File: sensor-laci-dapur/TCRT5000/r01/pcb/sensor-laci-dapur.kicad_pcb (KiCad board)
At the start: 2 copper layers, 66 x 14 mm, 8 parts

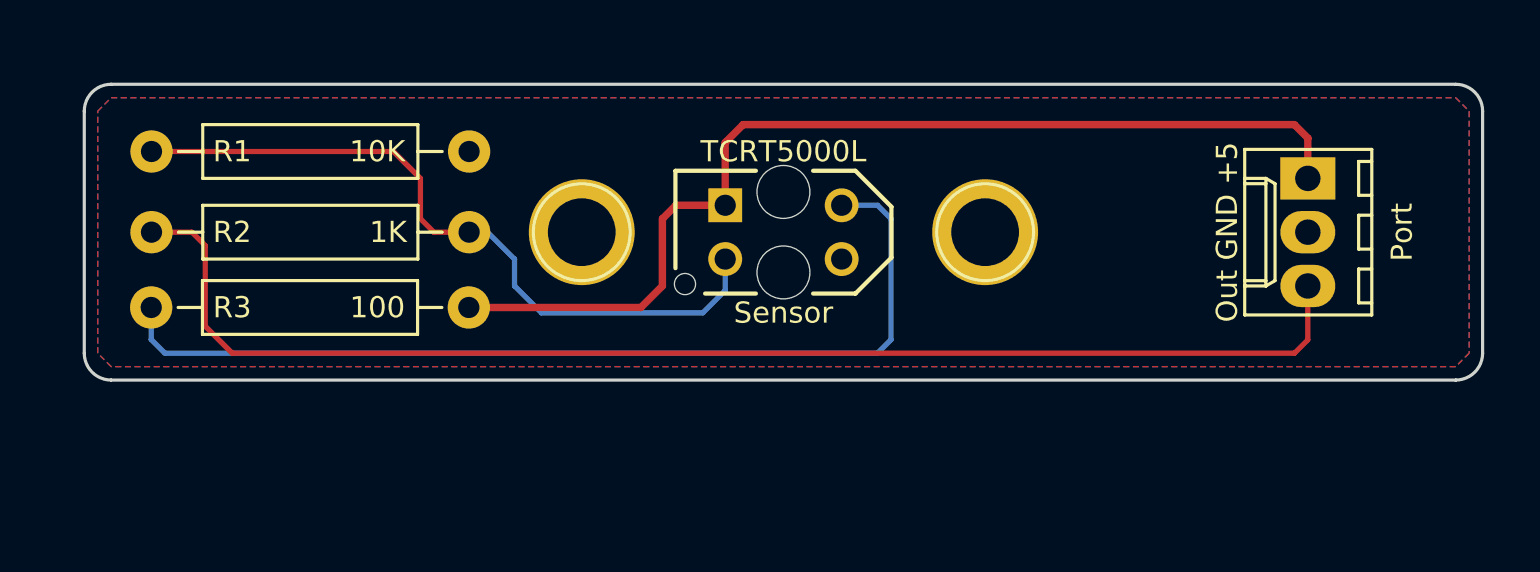
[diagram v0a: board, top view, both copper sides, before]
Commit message: Sensor Laci Dapur TCRT5000L rev01b
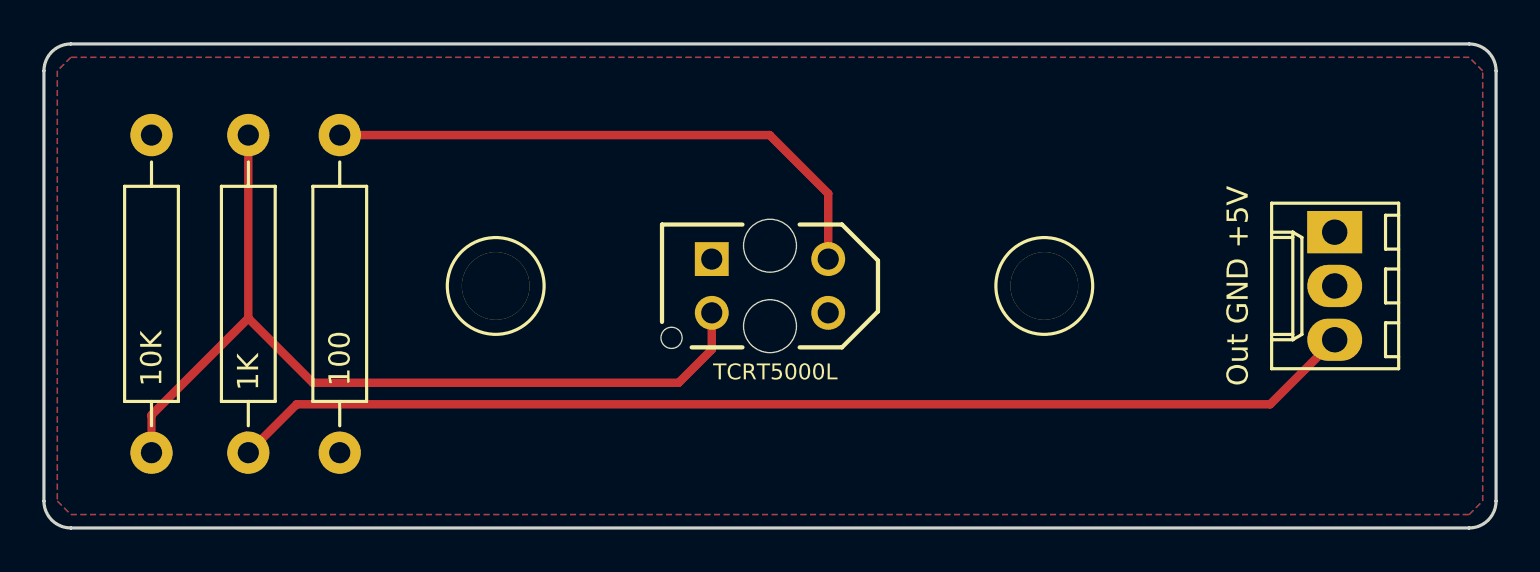
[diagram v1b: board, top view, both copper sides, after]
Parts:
- removed Port: Out GND +5, Connectors_Molex:Molex_KK-6410-03_03x2.54mm_Straight
- removed the REF** at (142.2, 95.2)
- removed the REF** at (161.3, 95.2)
- removed Sensor: TCRT5000L, TCRT5000L:XDCR_TCRT5000L
- added M: 1pin, Connect:1pin, F.Cu at (138.2, 97.8)
- added Port1: 1_Out, Connectors_Molex:Molex_KK-6410-03_03x2.54mm_Straight, F.Cu at (177.8, 95.2)
- added REF**: 1pin, Connect:1pin, F.Cu at (164.1, 97.8)
- added Sensor1: TCRT5000L, TCRT5000L:XDCR_TCRT5000L, F.Cu at (151.1, 97.8)
- moved REF** 43.3 mm to (126.5, 97.3)
- moved R1 14.2 mm to (121.9, 105.7), turned to 90 degrees
- moved R2 11.4 mm to (126.5, 105.7), turned to 90 degrees
- moved R3 9.18 mm to (130.8, 105.7), turned to 90 degrees
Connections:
- R1 pad 2: Net-(Port1-Pad2) -> /GND
- R2 pad 1: Net-(Port1-Pad3) -> /Out
- R3 pad 1: Net-(Port1-Pad1) -> /+5V
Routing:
- net Net-(Port1-Pad3): track 62.0 -> 0.00 mm
- net /Out: track 0.00 -> 53.9 mm
- net Net-(Port1-Pad1): track 49.0 -> 0.00 mm
- net Net-(R3-Pad2): track 45.3 -> 27.3 mm
- net Net-(R1-Pad1): track 34.6 -> 42.4 mm
- added copper zone on B.Cu, net /+5V
- added copper zone on F.Cu, net /GND
- removed copper zone on B.Cu, net Net-(Port1-Pad2)
- removed copper zone on F.Cu, net Net-(Port1-Pad2)
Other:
- board size 66 x 14 mm -> 68.6 x 22.9 mm
- net class +5 removed
- net class Default: clearance 0.2 -> 0.3; trace_width 0.25 -> 0.4
- net class Signal added: clearance 0.3, trace_width 0.4, via_dia 0.6, via_drill 0.4
- rule trace_clearance: 0.2 -> 0.3
- board text added: "Out GND +5V"
- board text added: "TCRT500L"
- board text added: "rev01"
